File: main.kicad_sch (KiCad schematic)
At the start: 0 parts

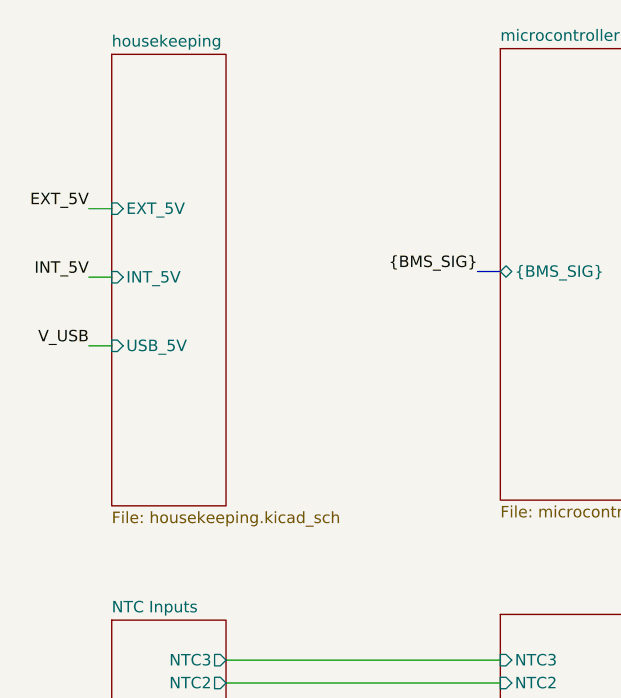
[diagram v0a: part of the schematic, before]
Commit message: Redoing layout
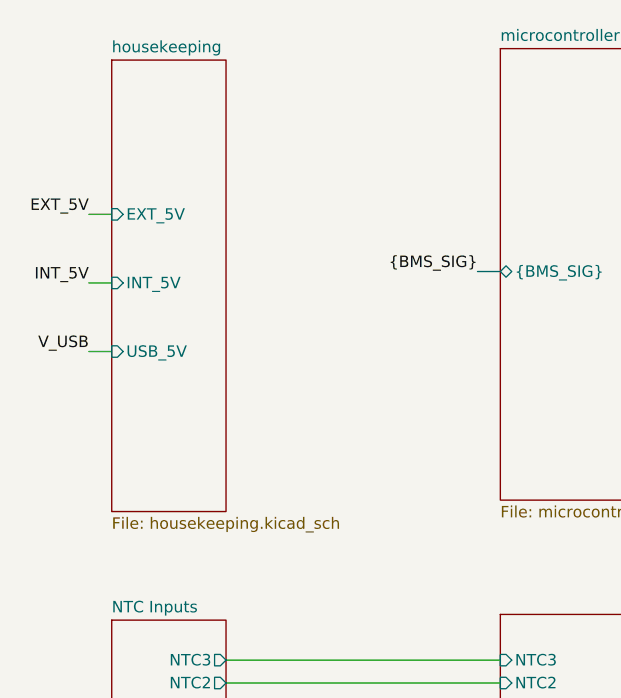
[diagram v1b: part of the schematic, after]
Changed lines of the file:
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@@
 	(wire
 		(pts
-			(xy 72.39 51.435) (xy 74.93 51.435)
+			(xy 72.39 52.07) (xy 74.93 52.07)
 		)
 		(stroke
@@
 	(wire
 		(pts
-			(xy 72.39 59.055) (xy 74.93 59.055)
+			(xy 72.39 59.69) (xy 74.93 59.69)
 		)
 		(stroke
@@
 	(wire
 		(pts
-			(xy 72.39 66.675) (xy 74.93 66.675)
+			(xy 72.39 67.31) (xy 74.93 67.31)
 		)
 		(stroke
@@
 	)
 	(label "V_USB"
-		(at 72.39 66.675 180)
+		(at 72.39 67.31 180)
 		(effects
 			(font
@@
 	)
 	(label "EXT_5V"
-		(at 72.39 51.435 180)
+		(at 72.39 52.07 180)
 		(effects
 			(font
@@
 	)
 	(label "INT_5V"
-		(at 72.39 59.055 180)
+		(at 72.39 59.69 180)
 		(effects
 			(font
@@
 	)
 	(sheet
-		(at 74.93 34.29)
+		(at 74.93 34.925)
 		(size 12.7 50.165)
 		(exclude_from_sim no)
@@
 		)
 		(property "Sheetname" "housekeeping"
-			(at 74.93 33.5784 0)
+			(at 74.93 34.2134 0)
 			(effects
 				(font
@@
 		)
 		(property "Sheetfile" "housekeeping.kicad_sch"
-			(at 74.93 85.0396 0)
+			(at 74.93 85.6746 0)
 			(effects
 				(font
@@
 		)
 		(pin "EXT_5V" input
-			(at 74.93 51.435 180)
+			(at 74.93 52.07 180)
 			(effects
 				(font
@@
 		)
 		(pin "INT_5V" input
-			(at 74.93 59.055 180)
+			(at 74.93 59.69 180)
 			(effects
 				(font
@@
 		)
 		(pin "USB_5V" input
-			(at 74.93 66.675 180)
-			(effects
-				(font
+			(at 74.93 67.31 180)
+			(effects
+				(font
